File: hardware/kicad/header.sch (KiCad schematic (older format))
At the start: 1 part, among them CN1 ADAFRUIT_FEATHER

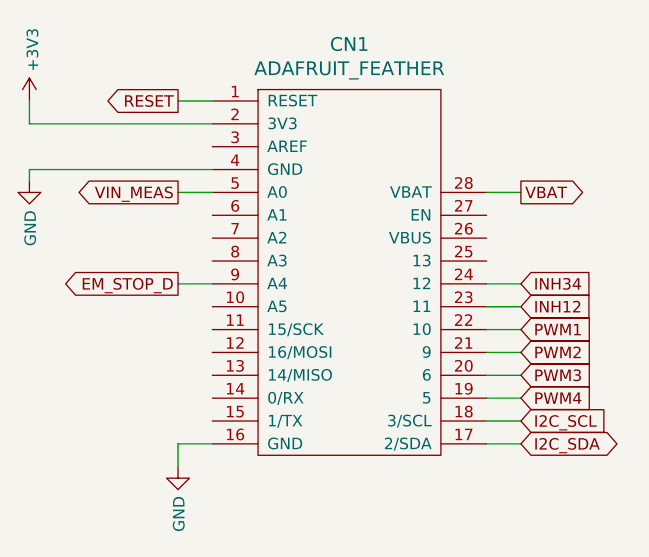
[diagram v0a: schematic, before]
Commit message: finished layout
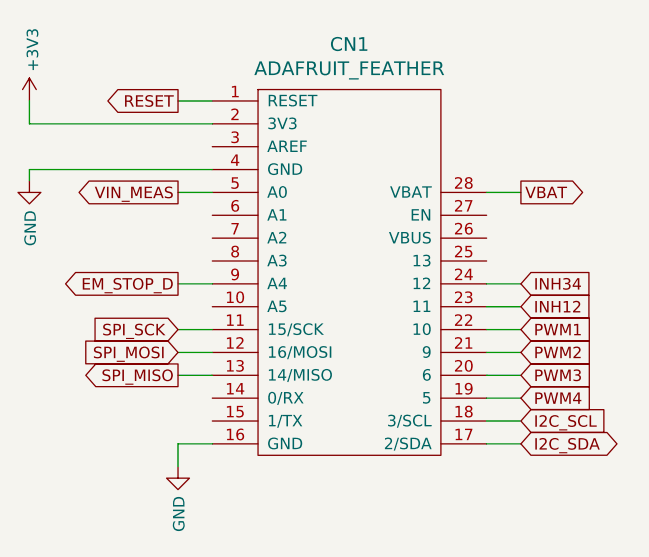
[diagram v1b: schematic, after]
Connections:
- net SPI_SCK: now reaches CN1.11 (15/SCK)
- net SPI_MOSI: now reaches CN1.12 (16/MOSI)
- net SPI_MISO: now reaches CN1.13 (14/MISO)
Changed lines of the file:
@@
 Wire Wire Line
 	4550 2950 5350 2950
+Text GLabel 5200 3950 0    50   Input ~ 0
+SPI_MOSI
+Text GLabel 5200 4050 0    50   Output ~ 0
+SPI_MISO
+Text GLabel 5200 3850 0    50   Input ~ 0
+SPI_SCK
+Wire Wire Line
+	5200 3850 5350 3850
+Wire Wire Line
+	5350 3950 5200 3950
+Wire Wire Line
+	5350 4050 5200 4050
 $EndSCHEMATC
